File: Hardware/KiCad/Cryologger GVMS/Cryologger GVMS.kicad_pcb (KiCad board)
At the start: 2 copper layers, 130.8 x 69.8 mm, 14 parts, among them J1 Screw_Terminal_01x02, J2 Screw_Terminal_01x02, U1 MMDLCB, U2 POLOLU_DV36, U3 GPS-RTK-SMA

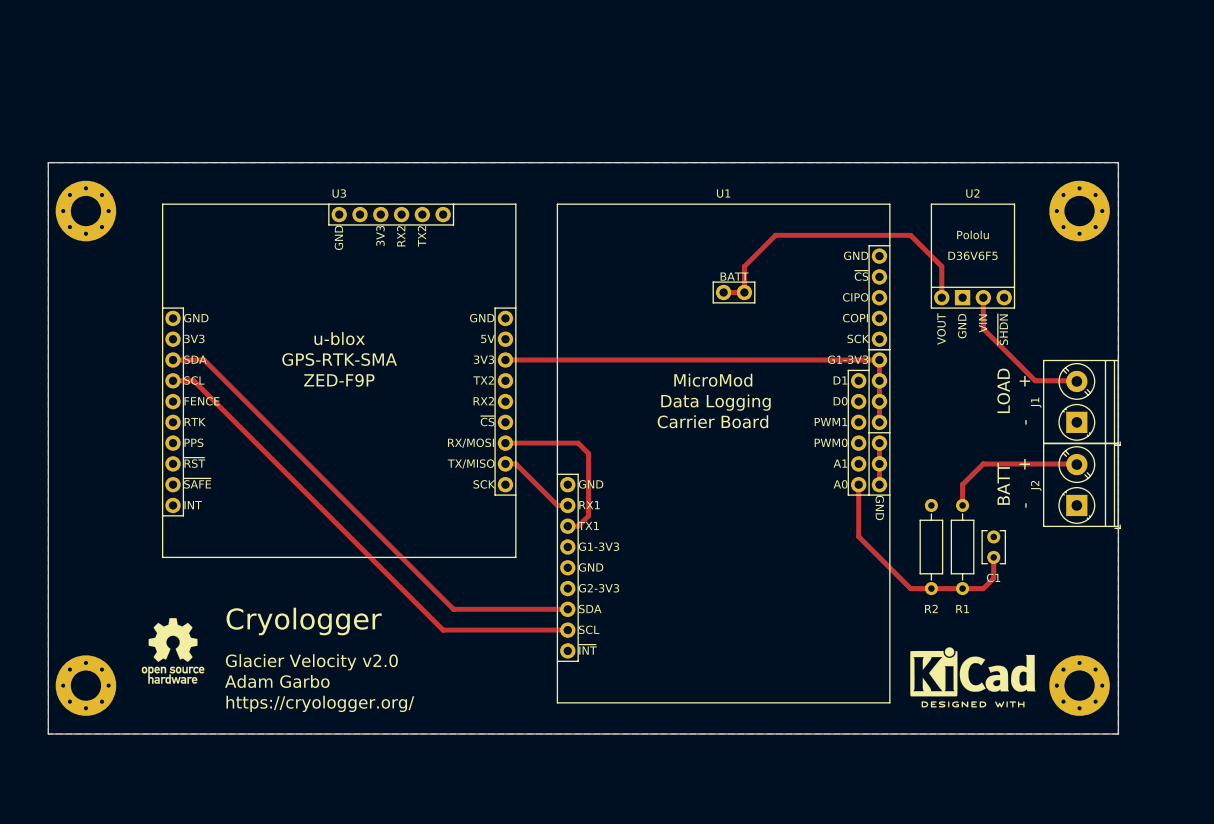
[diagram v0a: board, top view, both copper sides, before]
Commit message: Update KiCad files
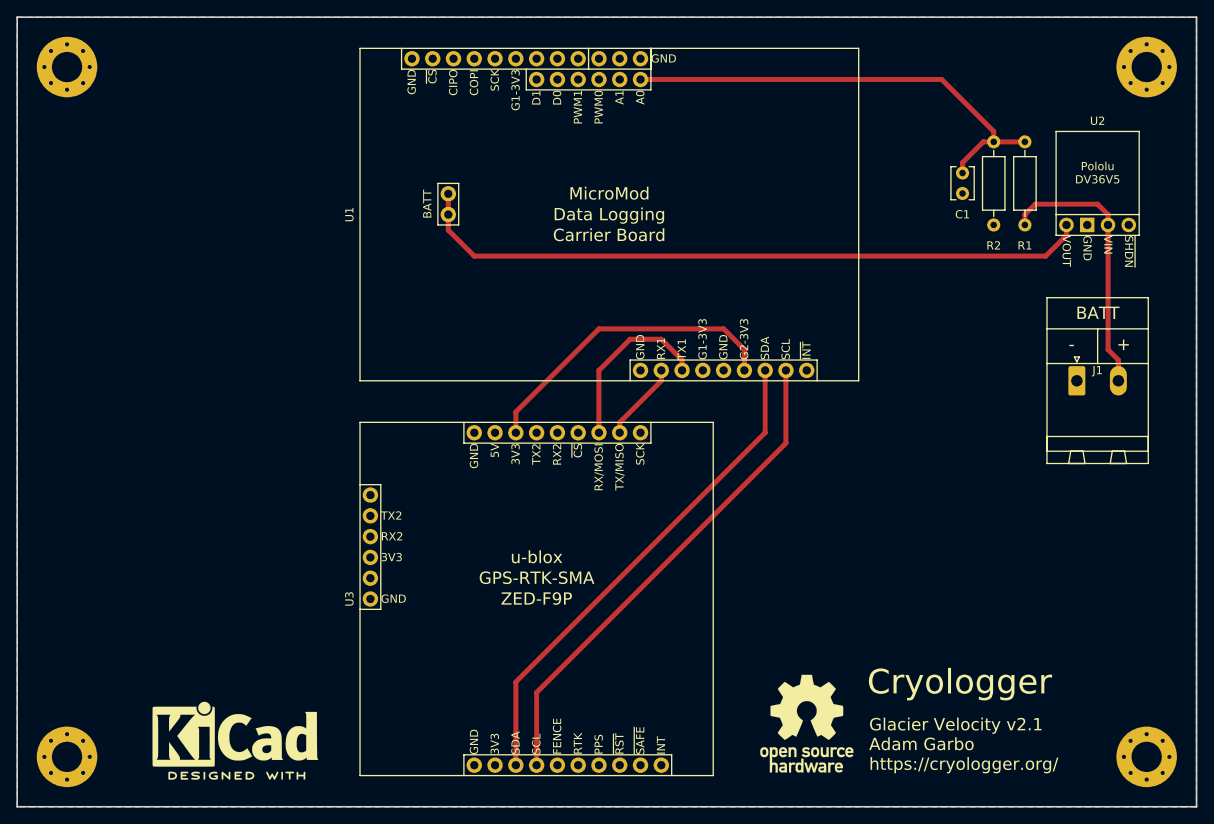
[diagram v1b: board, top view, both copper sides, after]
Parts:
- removed J2: Screw_Terminal_01x02, TerminalBlock_Phoenix:TerminalBlock_Phoenix_PT-1,5-2-5.0-H_1x02_P5.00mm_Horizontal
- removed the REF** at (83.8, 120.7)
- removed the REF** at (181.6, 123.2)
- added REF**: OSHW-Logo_11.4x12mm_SilkScreen, Symbol:OSHW-Logo_11.4x12mm_SilkScreen, F.Cu at (161.3, 129.5)
- added REF**: KiCad-Logo2_8mm_SilkScreen, Symbol:KiCad-Logo2_8mm_SilkScreen, F.Cu at (91.4, 130.8)
- J1: footprint TerminalBlock_Phoenix:TerminalBlock_Phoenix_PT-1,5-2-5.0-H_1x02_P5.00mm_Horizontal -> Connector_Phoenix_MSTB:PhoenixContact_MSTBA_2,5_2-G-5,08_1x02_P5.08mm_Horizontal
- U1: footprint Cryologger GVMS:MMDLCB -> Cryologger:SparkFun_MMDLCB
- U2: footprint Cryologger GVMS:POLOLU_DV36 -> Cryologger:Pololu_D36V6
- U3: footprint Cryologger GVMS:GPS-RTK-SMA -> Cryologger:SparkFun_GPS-RTK-SMA
- moved R2 55.1 mm to (184.2, 58.4), turned to 270 degrees
- moved C1 47.1 mm to (180.3, 62.2), turned to 270 degrees
- moved U3 36.0 mm to (128.3, 114.3), turned to 90 degrees
- moved R1 35.1 mm to (188.0, 68.6), turned to 90 degrees
- moved U1 32.4 mm to (137.2, 67.3), turned to 0 degrees
- moved H3 19.4 mm to (202.8, 49.3)
- moved H1 17.8 mm to (70.9, 49.3)
- moved U2 17.6 mm to (196.8, 63.5)
- moved H4 12.0 mm to (202.8, 133.6)
- moved H2 9.01 mm to (70.9, 133.6)
- moved J1 5.08 mm to (194.3, 87.6), turned to 0 degrees
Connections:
- net /VOUT renamed +5V
- J1 pad 2: /LOAD -> +BATT
- R1 pad 1: /VBAT -> +BATT
- U1 pad 10: Net-(U1-Pad10) -> (no net)
- U1 pad 11: Net-(U1-Pad11) -> (no net)
- U1 pad 12: Net-(U1-Pad12) -> (no net)
- U1 pad 13: Net-(U1-Pad13) -> (no net)
- U1 pad 14: Net-(U1-Pad14) -> (no net)
- U1 pad 15: /3V3 -> (no net)
- U1 pad 16: /3V3 -> (no net)
- U1 pad 17: /3V3 -> (no net)
- U1 pad 18: /3V3 -> (no net)
- U1 pad 22: Net-(U1-Pad22) -> (no net)
- U1 pad 23: Net-(U1-Pad23) -> (no net)
- U1 pad 24: Net-(U1-Pad24) -> (no net)
- U1 pad 25: Net-(U1-Pad25) -> (no net)
- U1 pad 26: Net-(U1-Pad26) -> (no net)
- U1 pad 4: Net-(U1-Pad4) -> (no net)
- U1 pad 6: Net-(U1-Pad6) -> +3V3
- U1 pad 9: Net-(U1-Pad9) -> (no net)
- U2 pad 3: /LOAD -> +BATT
- U2 pad 4: Net-(U2-Pad4) -> (no net)
- U3 pad 10: Net-(U3-Pad10) -> (no net)
- U3 pad 12: Net-(U3-Pad12) -> (no net)
- U3 pad 13: Net-(U3-Pad13) -> (no net)
- U3 pad 14: Net-(U3-Pad14) -> (no net)
- U3 pad 15: Net-(U3-Pad15) -> (no net)
- U3 pad 16: Net-(U3-Pad16) -> (no net)
- U3 pad 18: Net-(U3-Pad18) -> (no net)
- U3 pad 19: /3V3 -> +3V3
- U3 pad 2: Net-(U3-Pad2) -> (no net)
- U3 pad 20: Net-(U3-Pad20) -> (no net)
- U3 pad 21: Net-(U3-Pad21) -> (no net)
- U3 pad 22: Net-(U3-Pad22) -> (no net)
- U3 pad 25: Net-(U3-Pad25) -> (no net)
- U3 pad 5: Net-(U3-Pad5) -> (no net)
- U3 pad 6: Net-(U3-Pad6) -> (no net)
- U3 pad 7: Net-(U3-Pad7) -> (no net)
- U3 pad 8: Net-(U3-Pad8) -> (no net)
- U3 pad 9: Net-(U3-Pad9) -> (no net)
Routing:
- net /3V3: track 53.3 -> 0.00 mm
- net +5V: track 38.1 -> 83.6 mm
- net +3V3: track 0.00 -> 38.3 mm
- net +BATT: track 0.00 -> 34.6 mm
- net /A0: track 28.6 -> 57.0 mm
- net /LOAD: track 18.0 -> 0.00 mm
- net /VBAT: track 17.6 -> 0.00 mm
- net GND: track 5.08 -> 0.00 mm
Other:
- board size 130.8 x 69.8 mm -> 144.2 x 96.5 mm
- board text added: "Glacier Velocity v2.1 Adam Garbo https://cryologger.org/"
- board text added: "Pololu DV36V5"
- board text removed: "3V3"
- board text removed: "5V"
- board text removed: "A0"
- board text removed: "A1"
- board text removed: "Adam Garbo"
- board text removed: "CIPO"
- board text removed: "COPI"
- board text removed: "D0"
- board text removed: "D1"
- board text removed: "D36V6F5"
- board text removed: "Data Logging"
- board text removed: "FENCE"
- board text removed: "G1-3V3"
- board text removed: "G2-3V3"
- board text removed: "GND"
- board text removed: "GPS-RTK-SMA"
- board text removed: "Glacier Velocity v2.0"
- board text removed: "INT"
- board text removed: "LOAD"
- board text removed: "PPS"
- board text removed: "PWM0"
- board text removed: "PWM1"
- board text removed: "Pololu"
- board text removed: "RTK"
- board text removed: "RX/MOSI"
- board text removed: "RX1"
- board text removed: "RX2"
- board text removed: "SCK"
- board text removed: "SCL"
- board text removed: "SDA"
- board text removed: "TX/MISO"
- board text removed: "TX1"
- board text removed: "TX2"
- board text removed: "VIN"
- board text removed: "VOUT"
- board text removed: "https://cryologger.org/"
- board text removed: "u-blox"
- board text removed: "~CS"
- board text removed: "~INT"
- board text removed: "~RST"
- board text removed: "~SAFE"
- board text removed: "~SHDN"
